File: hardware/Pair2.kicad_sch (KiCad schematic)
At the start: 11 parts, among them IC3 TPS2HCS08AQPWPRQ1, J13 Conn_01x02, J5 Conn_01x02

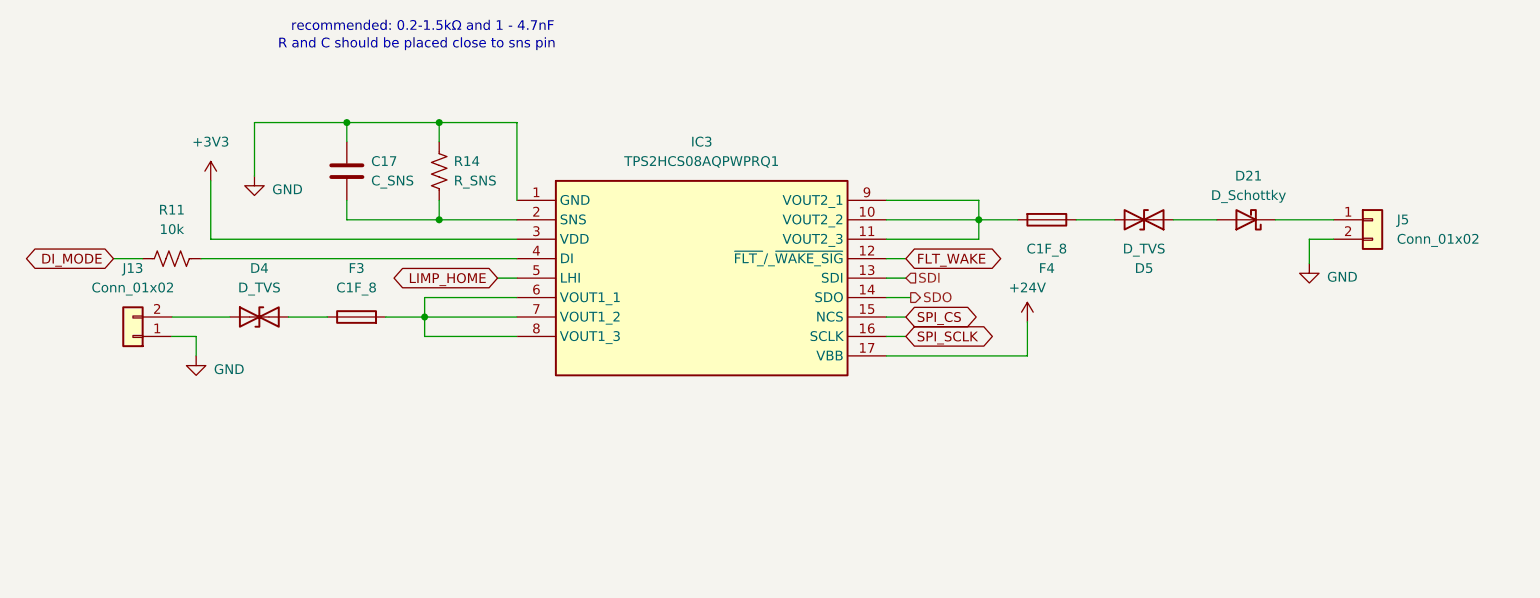
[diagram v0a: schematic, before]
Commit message: aesthetic added
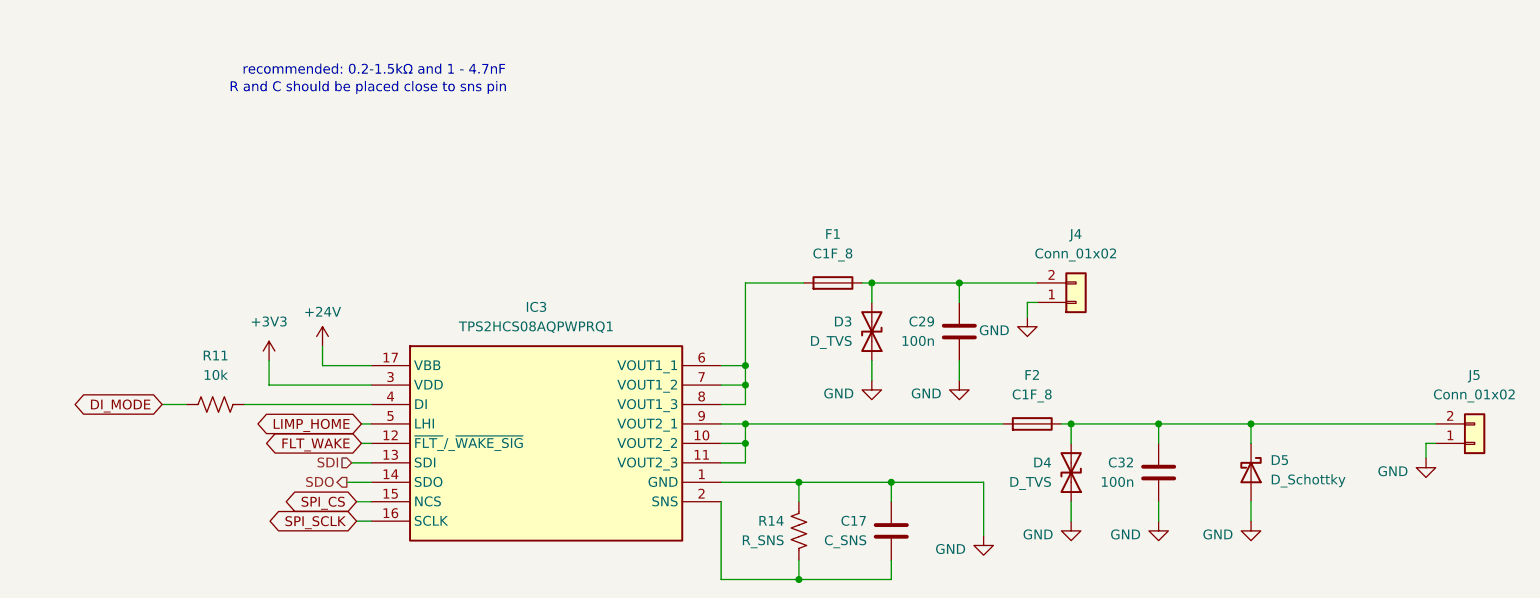
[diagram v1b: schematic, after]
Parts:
- removed D21: D_Schottky, symbol Device:D_Schottky
- removed D5: D_TVS, symbol Device:D_TVS
- removed F3, F4: C1F_8, Fuse:Fuse_1206_3216Metric, symbol PowerDistributionUnitLib:C1F_8
- removed J13: Conn_01x02, symbol Connector_Generic:Conn_01x02
- added C29, C32: 100n, symbol Device:C
- added D3: D_TVS, symbol Device:D_TVS
- added D5: D_Schottky, symbol Device:D_Schottky
- added F1, F2: C1F_8, Fuse:Fuse_1206_3216Metric, symbol PowerDistributionUnitLib:C1F_8
- added J4: Conn_01x02, symbol Connector_Generic:Conn_01x02
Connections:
- net GND: now also D4.1 (A1), J5.1 (Pin_1), C29.1, C32.1, D3.1 (A1), D5.2 (A), J4.1 (Pin_1); no longer J5.2 (Pin_2)
- net at IC3.10 (VOUT2_2), IC3.11 (VOUT2_3), IC3.9 (VOUT2_1): now also F2.2
- net at IC3.6 (VOUT1_1), IC3.7 (VOUT1_2), IC3.8 (VOUT1_3): now also F1.2
- net at D4.2 (A2): now also J5.2 (Pin_2), C32.2, D5.1 (K), F2.1
- new net: C29.2, D3.2 (A2), F1.1, J4.2 (Pin_2)
